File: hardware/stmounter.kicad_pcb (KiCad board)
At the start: 2 copper layers, 21 x 51 mm, 26 parts, among them J1 USB_C_Receptacle_USB2.0_14P, J2 Conn_01x20, J3 Conn_01x20, U1 STM32F103C8Tx, U2 SRV05-4, U3 AMS1117-3.3, Y1 16MHz 9pF, Y2 32.768kHz 12.5pF

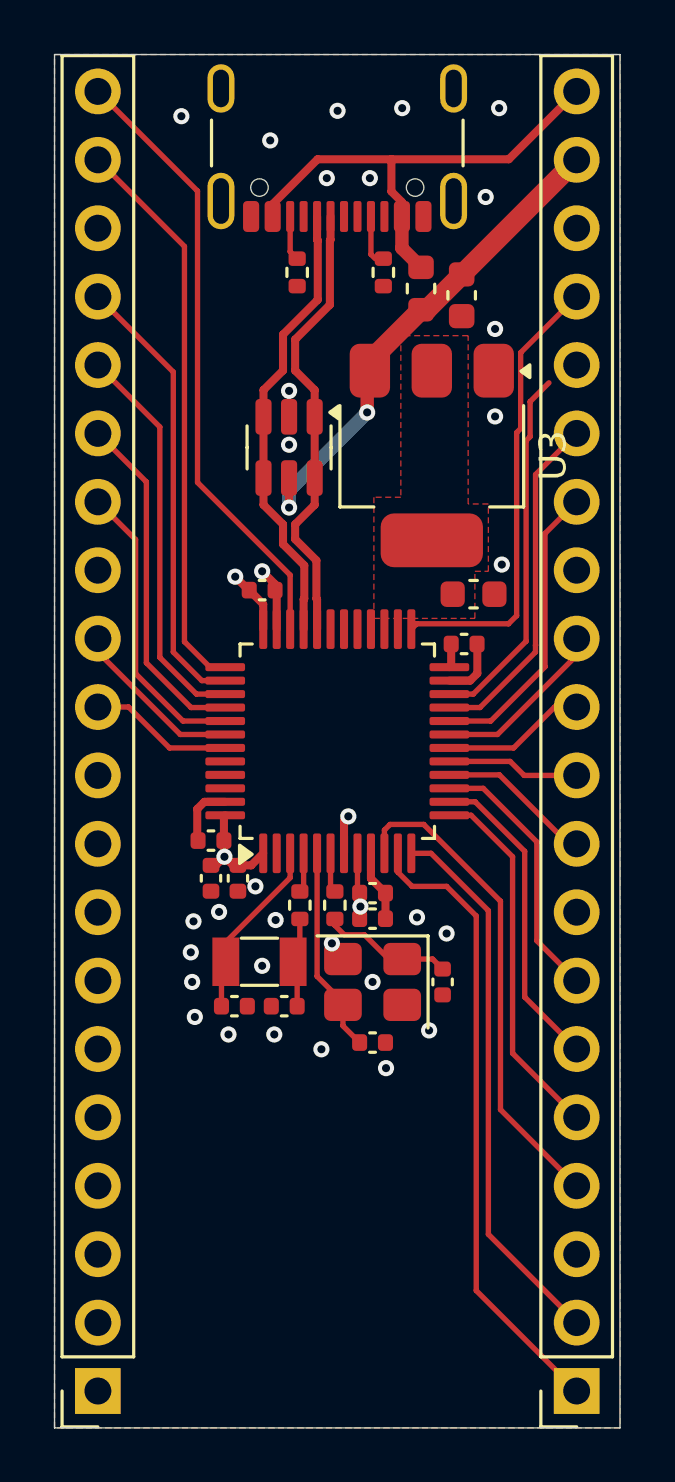
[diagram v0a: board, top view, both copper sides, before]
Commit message: Progress
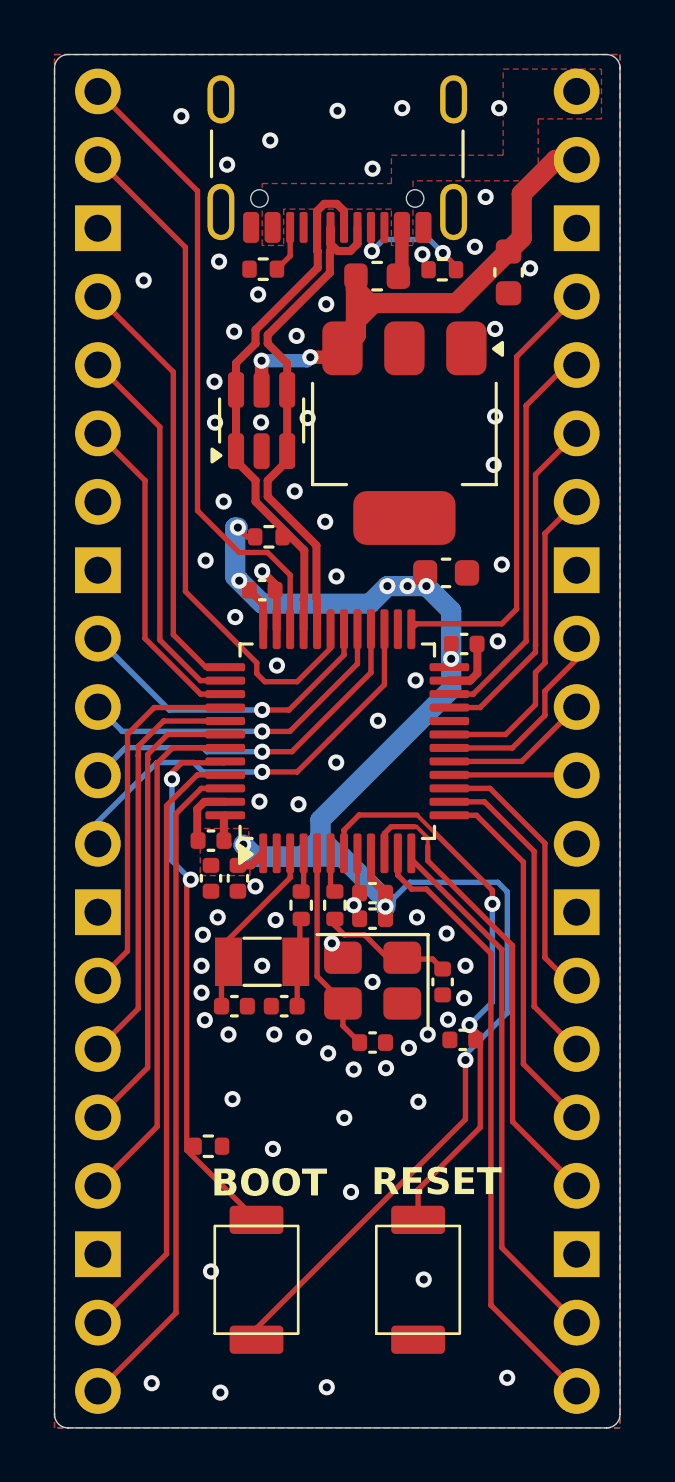
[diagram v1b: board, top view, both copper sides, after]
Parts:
- removed U1: STM32F103C8Tx, Package_QFP:LQFP-48_7x7mm_P0.5mm
- added C14: 100nF, Capacitor_SMD:C_0402_1005Metric, F.Cu at (163.6, 106.9)
- added R3: 1.5k, Resistor_SMD:R_0402_1005Metric, F.Cu at (156.3, 88.2)
- added R8: 10k, Resistor_SMD:R_0402_1005Metric, F.Cu at (154.1, 110.8)
- added SW1: SW_Push, stmounter:TS-1088-AR02016-Switch-SMD, F.Cu at (155.9, 115.8)
- added SW2: SW_Push, stmounter:TS-1088-AR02016-Switch-SMD, F.Cu at (161.9, 115.8)
- added U5: STM32F373CCTx, Package_QFP:LQFP-48_7x7mm_P0.5mm, F.Cu at (158.9, 95.8)
- C10, C11: value 10pF -> 15pF
- R5: value 390 -> 470
- Y1: value 16MHz 9pF -> 25MHz 12pF
- Y2: value 32.768kHz 12.5pF -> 32kHz 12.5pF
- moved R1 2.19 mm to (162.8, 78.3), turned to 180 degrees
- moved C2 1.94 mm to (165.2, 78.4)
- moved FB1 1.69 mm to (160.4, 78.5), turned to 180 degrees
- moved U2 1.43 mm to (156.1, 83.9), turned to 90 degrees
- moved U3 1.31 mm to (161.4, 84.4)
- moved C1 1.29 mm to (162.9, 89.6)
- moved R2 1.27 mm to (156.1, 78.3), turned to 0 degrees
- moved J1 0.41 mm to (158.9, 73.0)
- moved Y2 0.10 mm to (156.1, 104.0)
- moved R5 0.05 mm to (157.6, 101.9)
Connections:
- J1 pad S1: unconnected-(J1-SHIELD-PadS1) -> GND
- U2 pad 1: /D- -> /D+
- U2 pad 3: /D+ -> /D-
- U2 pad 4: /D+ -> /D-
- U2 pad 6: /D- -> /D+
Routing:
- net +3V3: track 9.89 -> 66.8 mm, vias 2 -> 9
- net /GPIO15: track 0.00 -> 24.9 mm
- net /GPIO14: track 0.00 -> 22.9 mm
- net Net-(U5-NRST): track 0.00 -> 21.5 mm, vias 0 -> 2
- net /BOOTSEL: track 0.00 -> 20.2 mm, vias 0 -> 2
- net /GPIO13: track 0.00 -> 19.4 mm
- net /GPIO12: track 0.00 -> 17.4 mm
- net VBUS: track 18.0 -> 1.86 mm
- net /GPIO9: track 0.00 -> 15.9 mm, vias 0 -> 1
- net /GPIO11: track 0.00 -> 15.5 mm
- net /GPIO10: track 0.00 -> 13.6 mm
- net /GPIO8: track 0.00 -> 13.5 mm, vias 0 -> 1
- net /GPIO5: track 11.0 -> 0.00 mm
- net /GPIO7: track 5.36 -> 12.3 mm, vias 0 -> 1
- net /GPIO22: track 5.79 -> 0.00 mm
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- added copper zone on F.Cu, net VBUS
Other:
- outline, holes or cut-outs redrawn
- board text added: "BOOT"
- board text added: "RESET"
